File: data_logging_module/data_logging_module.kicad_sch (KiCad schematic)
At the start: 6 parts, among them J1 Conn_01x15, J2 Conn_01x15

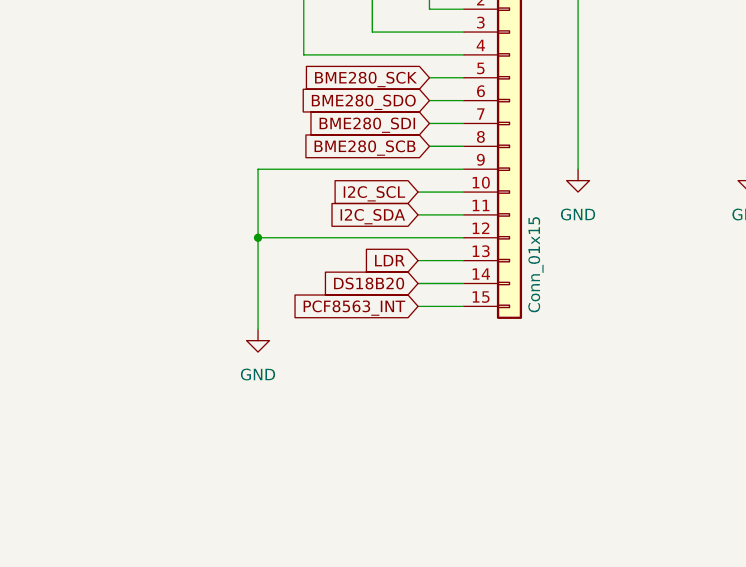
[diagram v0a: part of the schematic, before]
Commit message: initial PCB
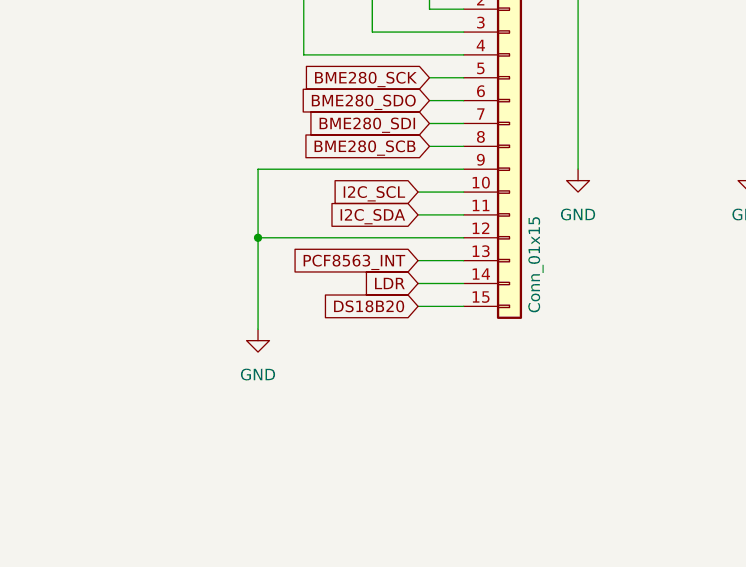
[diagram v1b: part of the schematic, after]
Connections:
- net DS18B20: now also J1.15 (Pin_15); no longer J1.14 (Pin_14)
- net LDR: now also J1.14 (Pin_14); no longer J1.13 (Pin_13)
- net PCF8563_INT: now also J1.13 (Pin_13); no longer J1.15 (Pin_15)
